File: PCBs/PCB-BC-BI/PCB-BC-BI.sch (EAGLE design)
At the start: 21 parts, among them U1 ARDUINO_SHIELDBOXSHIELD

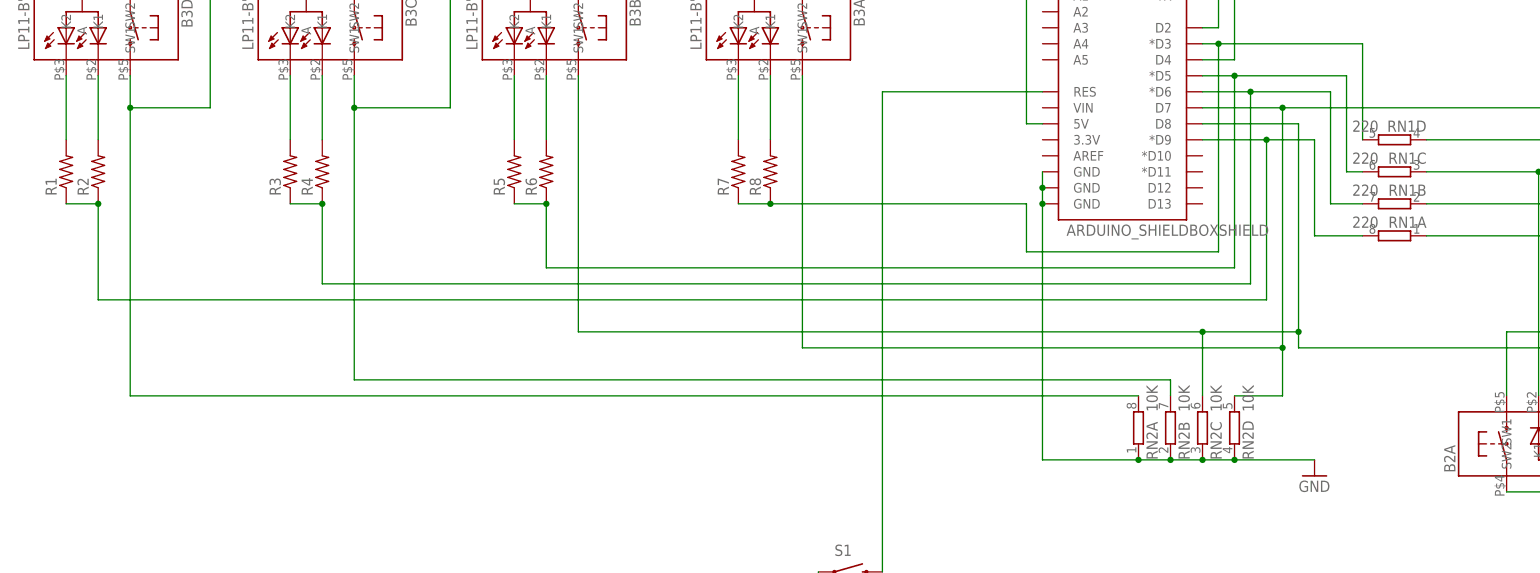
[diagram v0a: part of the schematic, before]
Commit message: asdf
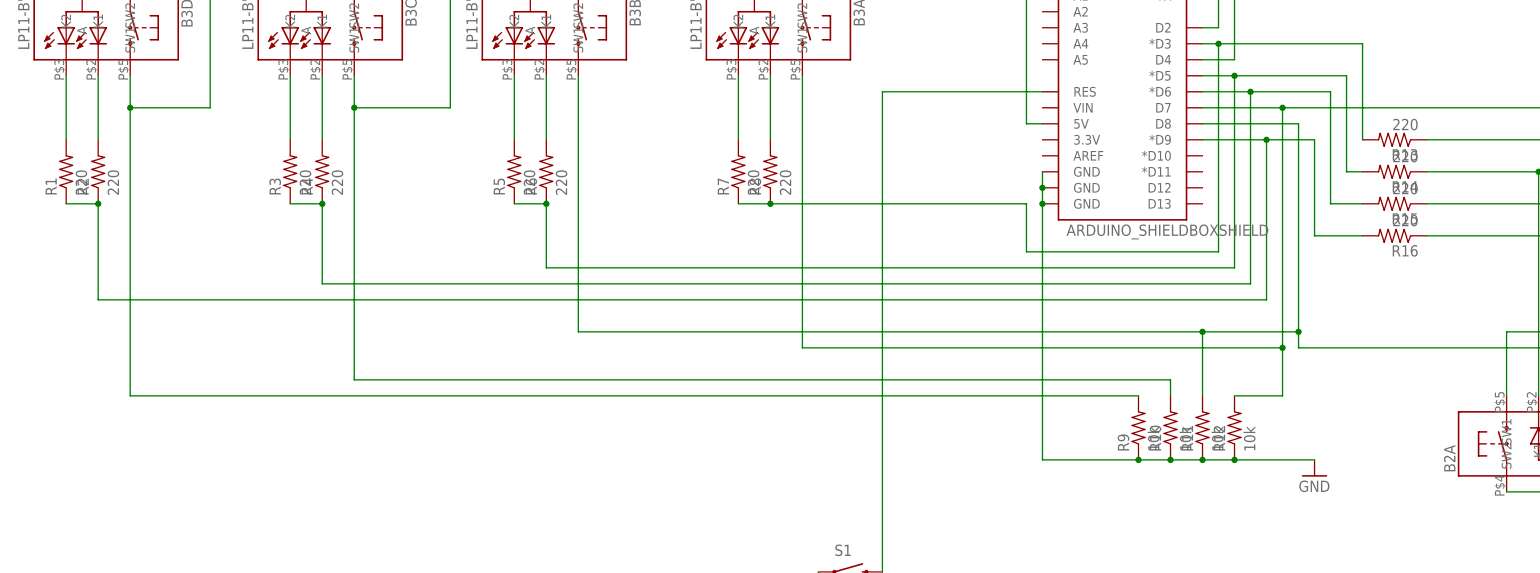
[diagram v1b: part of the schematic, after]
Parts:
- removed RN1: 220, resistor-dil:4R-NCAY16
- removed RN2: 10K, resistor-dil:4R-NCAY16
- added R10, R11, R12, R9: 10k, SparkFun:RESISTOR0603-RES
- added R13, R14, R15, R16: 220, SparkFun:RESISTOR0603-RES
- R1, R2, R3, R4, R5, R6, R7, R8: value (none) -> 220
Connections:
- net GND: now also R10.1, R11.1, R12.1, R9.1; no longer RN2A.1, RN2B.1, RN2C.1, RN2D.1
- net N$10: now also R16.2; no longer RN1A.2
- net N$11: now also R11.2; no longer RN2C.2
- net N$12: now also R14.1; no longer RN1C.1
- net N$13: now also R15.1; no longer RN1B.1
- net N$14: now also R16.1; no longer RN1A.1
- net N$15: now also R12.2; no longer RN2D.2
- net N$20: now also R9.2; no longer RN2A.2
- net N$21: now also R13.2; no longer RN1D.2
- net N$3: now also R13.1; no longer RN1D.1
- net N$7: now also R10.2; no longer RN2B.2
- net N$8: now also R14.2; no longer RN1C.2
- net N$9: now also R15.2; no longer RN1B.2
